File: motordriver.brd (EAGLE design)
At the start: 101.3 x 82.5 mm, 98 parts, among them J1 CONNECTOR_MOTORS, J10 HEADER_1X3, J11 HEADER_1X3, J2 CONNECTOR_MOTORS, J3 CONNECTOR_MOTORS, J4 CONNECTOR_MOTORS, J5 HEADER_1X3, J6 HEADER_1X3, J7 HEADER_1X3, J8 HEADER_1X3, J9 CONNECTOR_MOTORS, Q1 MOSFET, Q10 MOSFET, Q11 MOSFET, Q12 MOSFET, Q13 MOSFET, Q14 MOSFET, Q15 MOSFET, Q16 MOSFET, Q2 MOSFET, Q3 MOSFET, Q4 MOSFET, Q5 MOSFET, Q6 MOSFET, Q7 MOSFET, Q8 MOSFET, Q9 MOSFET, U1 74XX139_PDIP, U10 IR2111_PDIP, U11 IR2111_PDIP, U12 7812_TO220, U2 TL084_PDIP, U3 7812_TO220, U4 IR2111_PDIP, U5 IR2111_PDIP, U6 IR2111_PDIP, U7 IR2111_PDIP, U8 IR2111_PDIP, U9 IR2111_PDIP

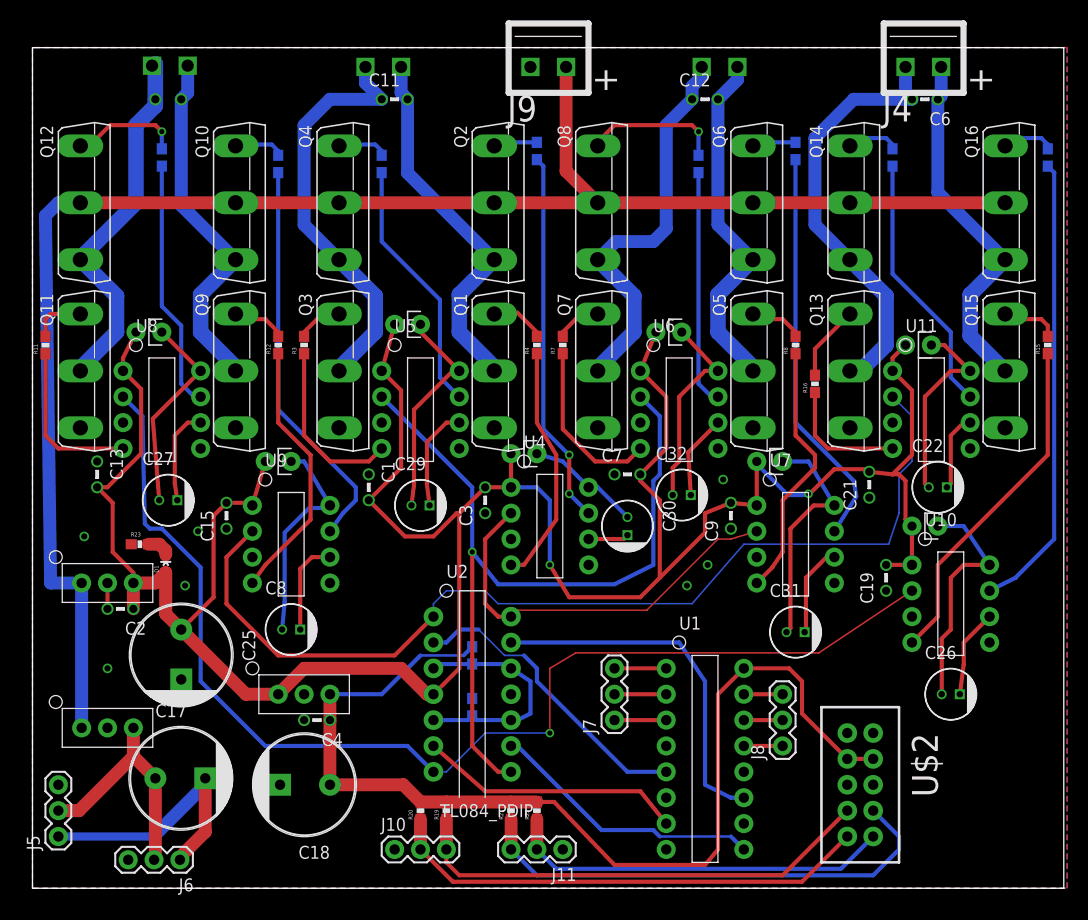
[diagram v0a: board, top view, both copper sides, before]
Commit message: Front side labels...COMPLETE
IT tAkes AlOT of COoKs to mAke A STew.
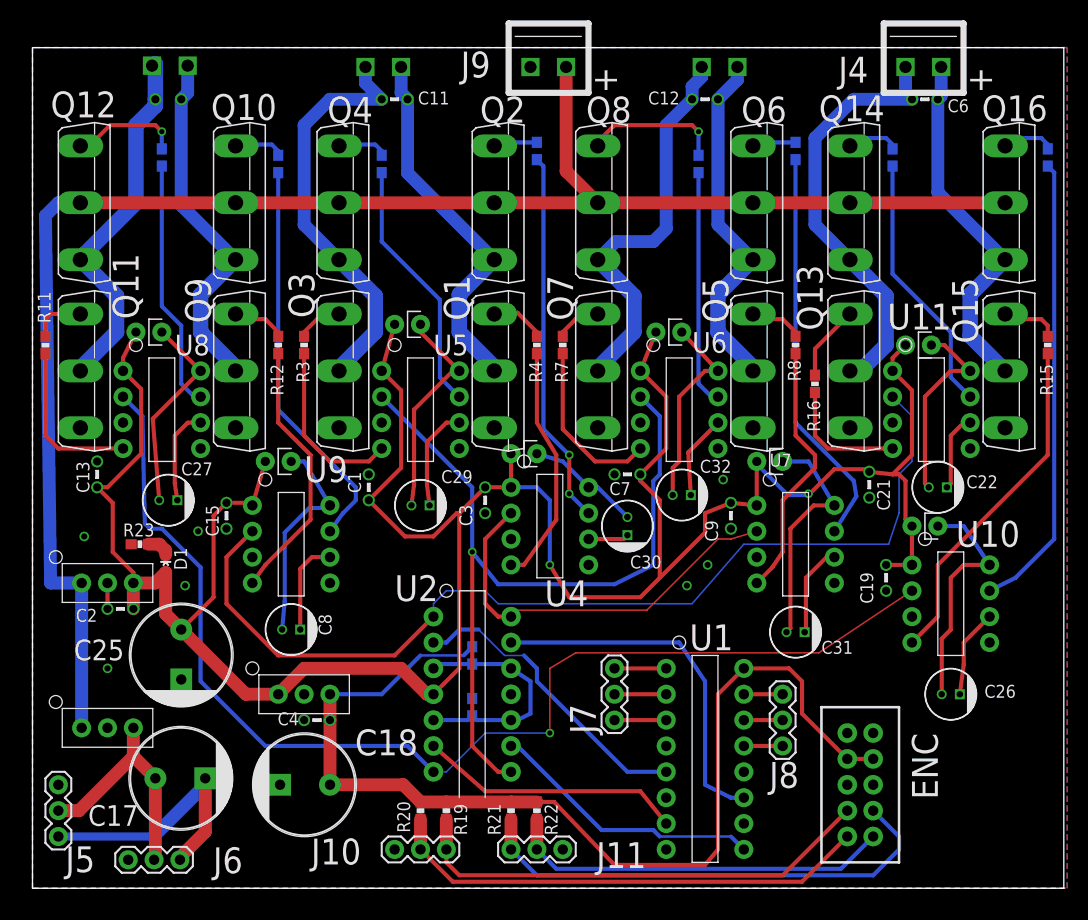
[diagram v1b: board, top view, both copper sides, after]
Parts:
- renumbered U$2 to ENC
